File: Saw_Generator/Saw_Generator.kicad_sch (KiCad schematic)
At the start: 1 part

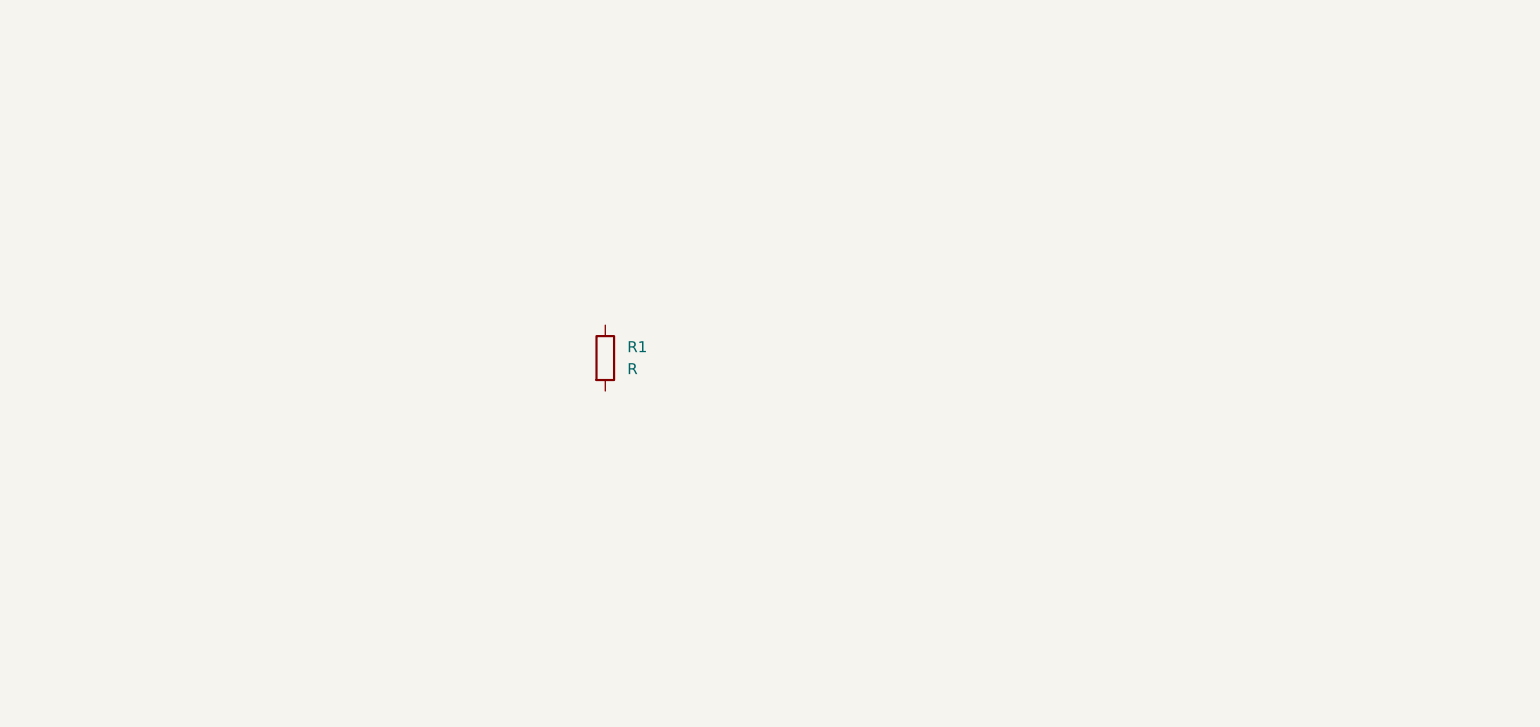
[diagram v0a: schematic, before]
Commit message: saw generator
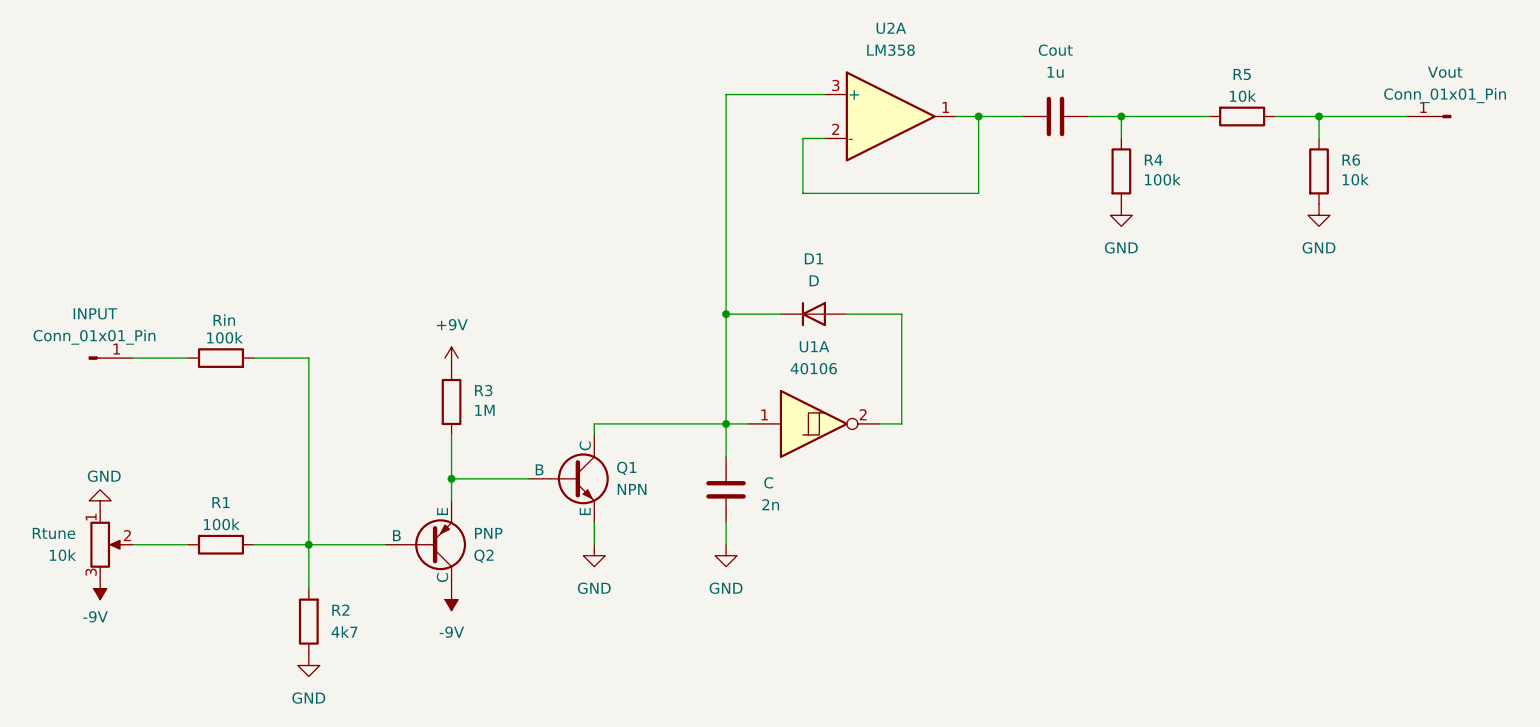
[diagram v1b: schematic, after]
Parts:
- added C: 2n, symbol Device:C
- added Cout: 1u, symbol Device:C
- added D1: D, symbol Device:D
- added INPUT, Vout: Conn_01x01_Pin, symbol Connector:Conn_01x01_Pin
- added Q1: NPN, symbol Simulation_SPICE:NPN
- added Q2: PNP, symbol Simulation_SPICE:PNP
- added R2: 4k7, symbol Device:R
- added R3: 1M, symbol Device:R
- added R4, Rin: 100k, symbol Device:R
- added R5, R6: 10k, symbol Device:R
- added Rtune: 10k, symbol Device:R_Potentiometer
- added U1: 40106, symbol 4xxx:40106
- added U2: LM358, symbol Amplifier_Operational:LM358
- R1: value R -> 100k
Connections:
- net at R1.1: now also Q2.2 (B), R2.2, Rin.2
- net at R1.2: now also Rtune.2
- new net: R5.1, R6.1, Vout.1 (Pin_1)
- new net: Cout.1, U2.1, U2.2 (-)
- new net: C.1, D1.1 (K), Q1.1 (C), U1.1, U2.3 (+)
- new net: Cout.2, R4.1, R5.2
- new net: D1.2 (A), U1.2
- new net: Q1.2 (B), Q2.3 (E), R3.2
- new net: INPUT.1 (Pin_1), Rin.1
- new net +9V: R3.1
- new net -9V: Q2.1 (C), Rtune.3
- new net GND: C.2, Q1.3 (E), R2.1, R4.2, R6.2, Rtune.1
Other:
- moved on the sheet: R1
